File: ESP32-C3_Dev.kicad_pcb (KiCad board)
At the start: 2 copper layers, 32.7 x 47.2 mm, 103 parts, among them J4 USB_C_Receptacle_USB2.0_16P, J5 Conn_01x03_Socket, J6 Conn_01x03_Socket, J8 Conn_01x02_Pin, Q1 Dual_NMOS_8205A, SW1 SW_MEC_5G, SW2 SW_MEC_5G, U1 ESP32-C3-WROOM-02, U2 AMS1117-3.3, U3 DW01A, U4 TLV9002S, U5 OLED_SSD1306, U6 TP4056, U8 BMP388, U9 XC6220B181MR

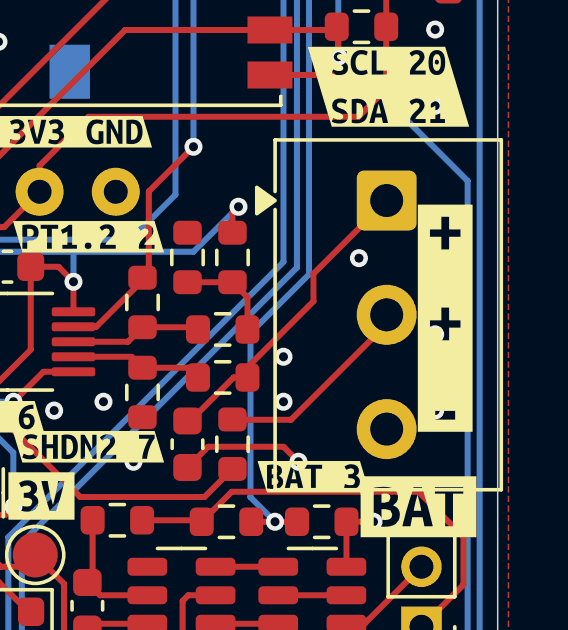
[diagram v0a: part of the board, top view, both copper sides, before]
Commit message: wip
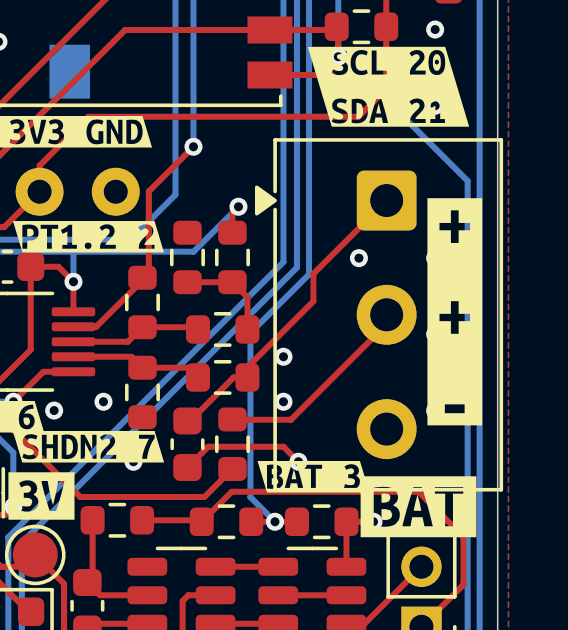
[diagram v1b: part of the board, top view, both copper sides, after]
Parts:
- moved kibuzzard-68E98378 0.39 mm to (155.7, 79.5)
- moved kibuzzard-68EE7E42 0.21 mm to (155.7, 79.5)
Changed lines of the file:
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@@
 	(footprint "kibuzzard-68E98378"
 		(layer "F.Cu")
-		(at 155.391151 79.715915)
+		(at 155.71 79.5)
 		(descr "Generated with KiBuzzard")
 		(tags "kb_params=eyJBbGlnbm1lbnRDaG9pY2UiOiAiQ2VudGVyIiwgIkNhcExlZnRDaG9pY2UiOiAiWyIsICJDYXBSaWdodENob2ljZSI6ICJdIiwgIkZvbnRDb21ib0JveCI6ICJVYnVudHVNb25vLUIiLCAiSGVpZ2h0Q3RybCI6IDEuNSwgIkxheWVyQ29tYm9Cb3giOiAiRi5TaWxrUyIsICJMaW5lU3BhY2luZ0N0cmwiOiAxLjUsICJNdWx0aUxpbmVUZXh0IjogIitcclxuK1xyXG4tIiwgIlBhZGRpbmdCb3R0b21DdHJsIjogMi4wLCAiUGFkZGluZ0xlZnRDdHJsIjogMi4wLCAiUGFkZGluZ1JpZ2h0Q3RybCI6IDIuMCwgIlBhZGRpbmdUb3BDdHJsIjogMi4wLCAiV2lkdGhDdHJsIjogMC4wLCAiYWR2YW5jZWRDaGVja2JveCI6IGZhbHNlLCAiaW5saW5lRm9ybWF0VGV4dGJveCI6IGZhbHNlLCAibGluZW92ZXJTdHlsZUNob2ljZSI6ICJTcXVhcmUiLCAibGluZW92ZXJUaGlja25lc3NDdHJsIjogMX0=")
@@
 	(footprint "kibuzzard-68EE7E42"
 		(layer "B.Cu")
-		(at 155.5 79.5 180)
+		(at 155.71 79.5 180)
 		(descr "Generated with KiBuzzard")
 		(tags "kb_params=eyJBbGlnbm1lbnRDaG9pY2UiOiAiQ2VudGVyIiwgIkNhcExlZnRDaG9pY2UiOiAiWyIsICJDYXBSaWdodENob2ljZSI6ICJdIiwgIkZvbnRDb21ib0JveCI6ICJVYnVudHVNb25vLUIiLCAiSGVpZ2h0Q3RybCI6IDEuNSwgIkxheWVyQ29tYm9Cb3giOiAiRi5TaWxrUyIsICJMaW5lU3BhY2luZ0N0cmwiOiAxLjUsICJNdWx0aUxpbmVUZXh0IjogIi1cclxuK1xyXG4rIiwgIlBhZGRpbmdCb3R0b21DdHJsIjogMi4wLCAiUGFkZGluZ0xlZnRDdHJsIjogMi4wLCAiUGFkZGluZ1JpZ2h0Q3RybCI6IDIuMCwgIlBhZGRpbmdUb3BDdHJsIjogMi4wLCAiV2lkdGhDdHJsIjogMC4wLCAiYWR2YW5jZWRDaGVja2JveCI6IGZhbHNlLCAiaW5saW5lRm9ybWF0VGV4dGJveCI6IGZhbHNlLCAibGluZW92ZXJTdHlsZUNob2ljZSI6ICJTcXVhcmUiLCAibGluZW92ZXJUaGlja25lc3NDdHJsIjogMX0=")
